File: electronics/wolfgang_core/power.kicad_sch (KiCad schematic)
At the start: 25 parts, among them J1 Battery, J2 Power Supply, U1 LM5001MA, U2 ACS724xLCTR-50AB, U3 LTC4418IUF-PBF

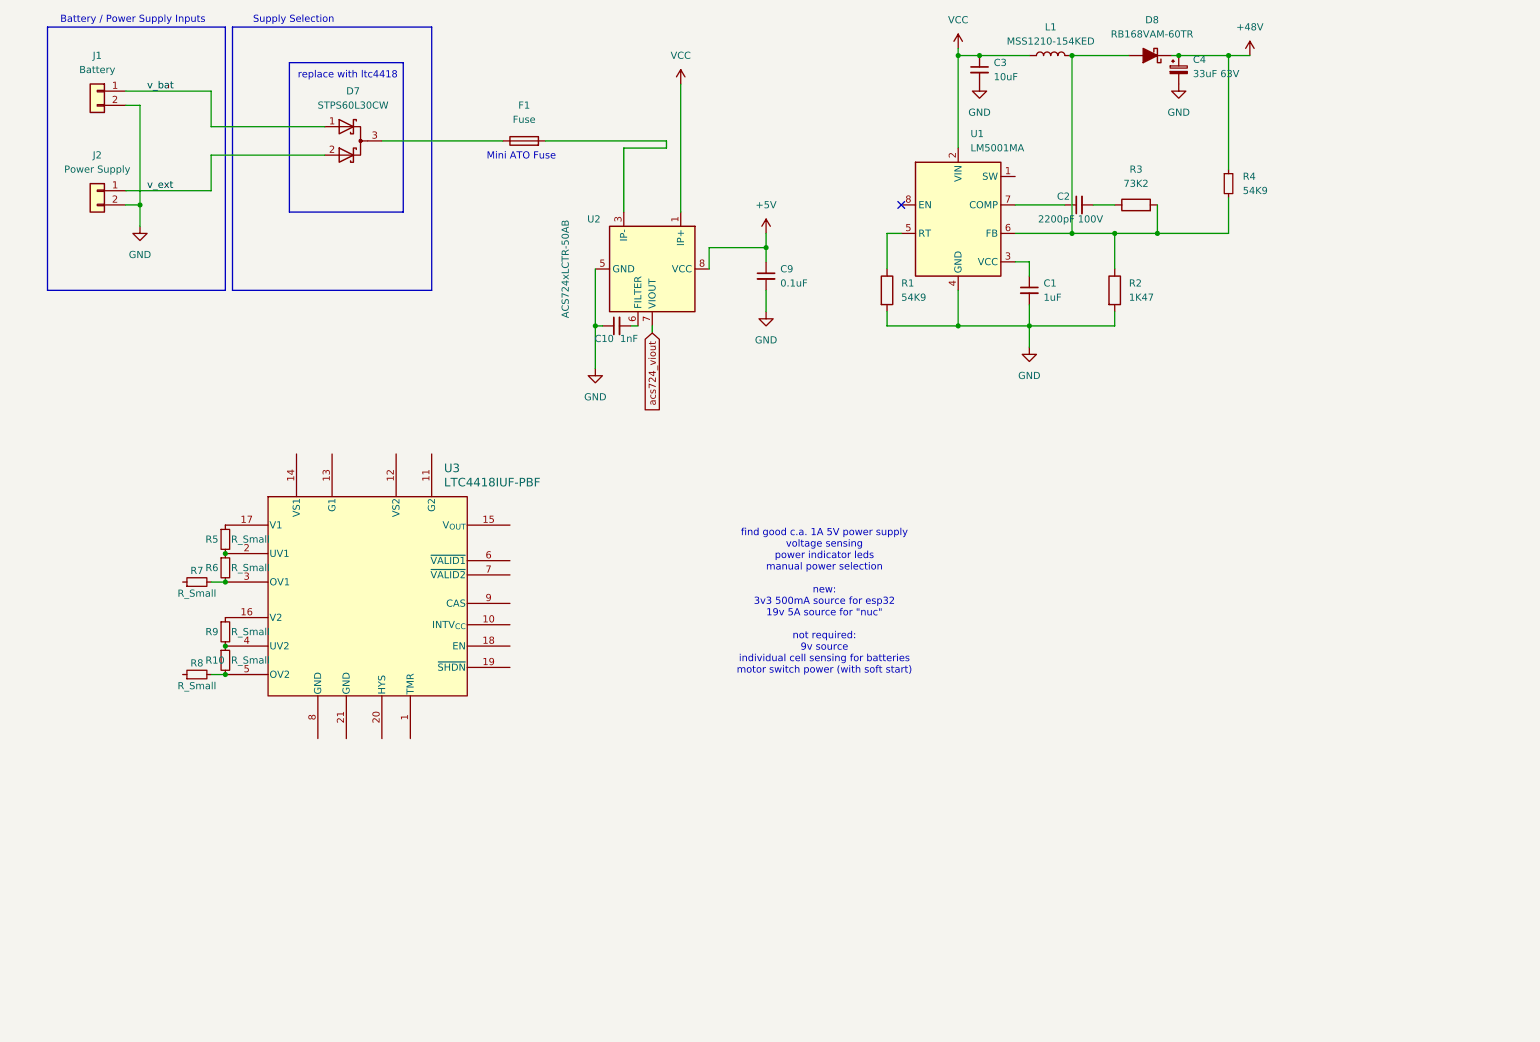
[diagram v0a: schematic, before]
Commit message: More work on CORE Rev2
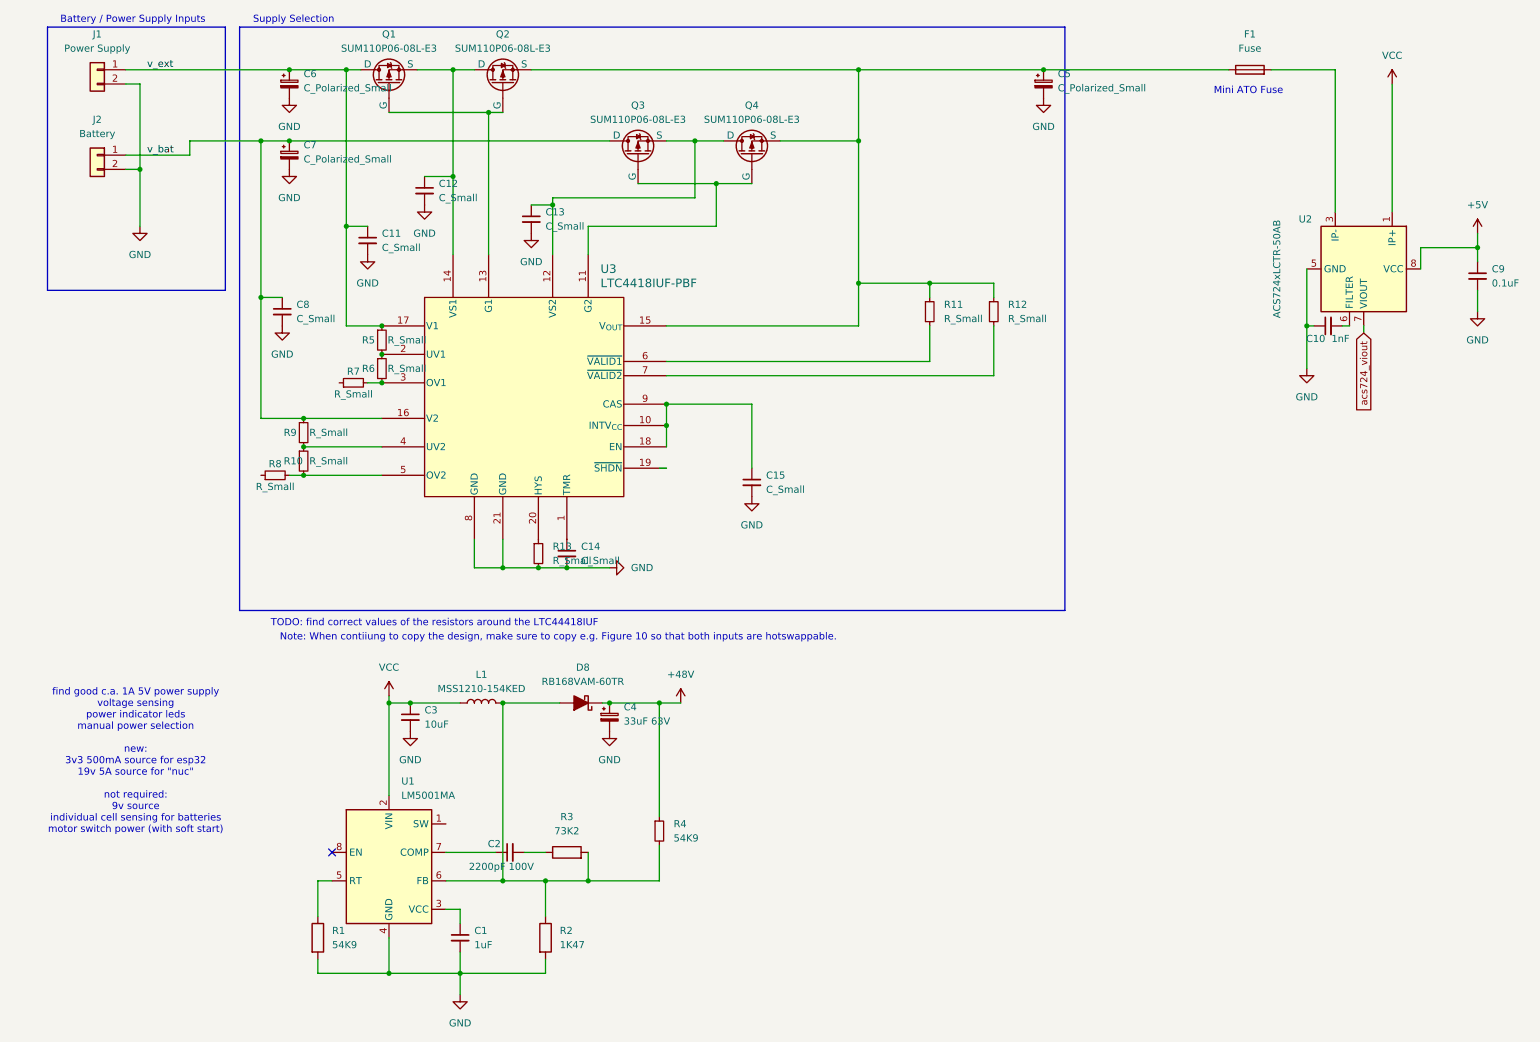
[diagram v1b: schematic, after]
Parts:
- removed D7: STPS60L30CW, symbol Device:D_Schottky_Dual_CommonCathode_AAK_Parallel
- added C11, C12, C13, C14, C15, C8: C_Small, symbol Device:C_Small
- added C5, C6, C7: C_Polarized_Small, symbol Device:C_Polarized_Small
- added Q1, Q2, Q3, Q4: SUM110P06-08L-E3, symbol Simulation_SPICE:PMOS
- added R11, R12, R13: R_Small, symbol Device:R_Small
- renumbered J2 to J1, J1 to J2
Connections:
- net GND: now also U3.21 (GND), U3.8 (GND), C11.2, C12.2, C13.2, C14.2, C15.2, C5.2, C6.2, C7.2, C8.2, R13.2
- net v_bat: now also R9.1, U3.16 (V2), C7.1, C8.1, Q3.1 (D)
- net v_ext: now also R5.1, U3.17 (V1), C11.1, C6.1, Q1.1 (D)
- net at F1.1: now also U3.15 (V_{OUT}), C5.1, Q2.3 (S), Q4.3 (S), R11.1, R12.1
- net at U3.1 (TMR): now also C14.1
- net at U3.10 (INTV_{CC}): now also U3.18 (EN), U3.9 (CAS), C15.1
- net at U3.11 (G2): now also Q3.2 (G), Q4.2 (G)
- net at U3.12 (VS2): now also C13.1, Q3.3 (S), Q4.1 (D)
- net at U3.13 (G1): now also Q1.2 (G), Q2.2 (G)
- net at U3.14 (VS1): now also C12.1, Q1.3 (S), Q2.1 (D)
- net at U3.20 (HYS): now also R13.1
- net at U3.6 (~{VALID1}): now also R11.2
- net at U3.7 (~{VALID2}): now also R12.2
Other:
- note added: "Note: When contiiung to copy the design, make sure to copy e.g. Figure 10 so that both inputs are hotswappable."
- note added: "TODO: find correct values of the resistors around the LTC44418IUF"
- note removed: "replace with ltc4418"
- moved on the sheet: C1, C10, C2, C3, C4, C9, D8, F1, J1, J2, L1, R1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
